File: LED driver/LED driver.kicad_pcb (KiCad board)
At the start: 2 copper layers, 65 x 45 mm, 49 parts, among them J1 Conn_VCC, J2 Conn_LED, J3 Conn_Aux, J4 Conn_UART, J5 PWR_AUX, Q1 ZXMN3A01F, Q2 ZXMN3A01F, Q3 ZXMN3A01F, Q4 ZXMN3A01F, Q5 ZXMN3A01F, SW1 SW_Push, U1 ESP32-C3-MINI-1-N4, U2 MP2359

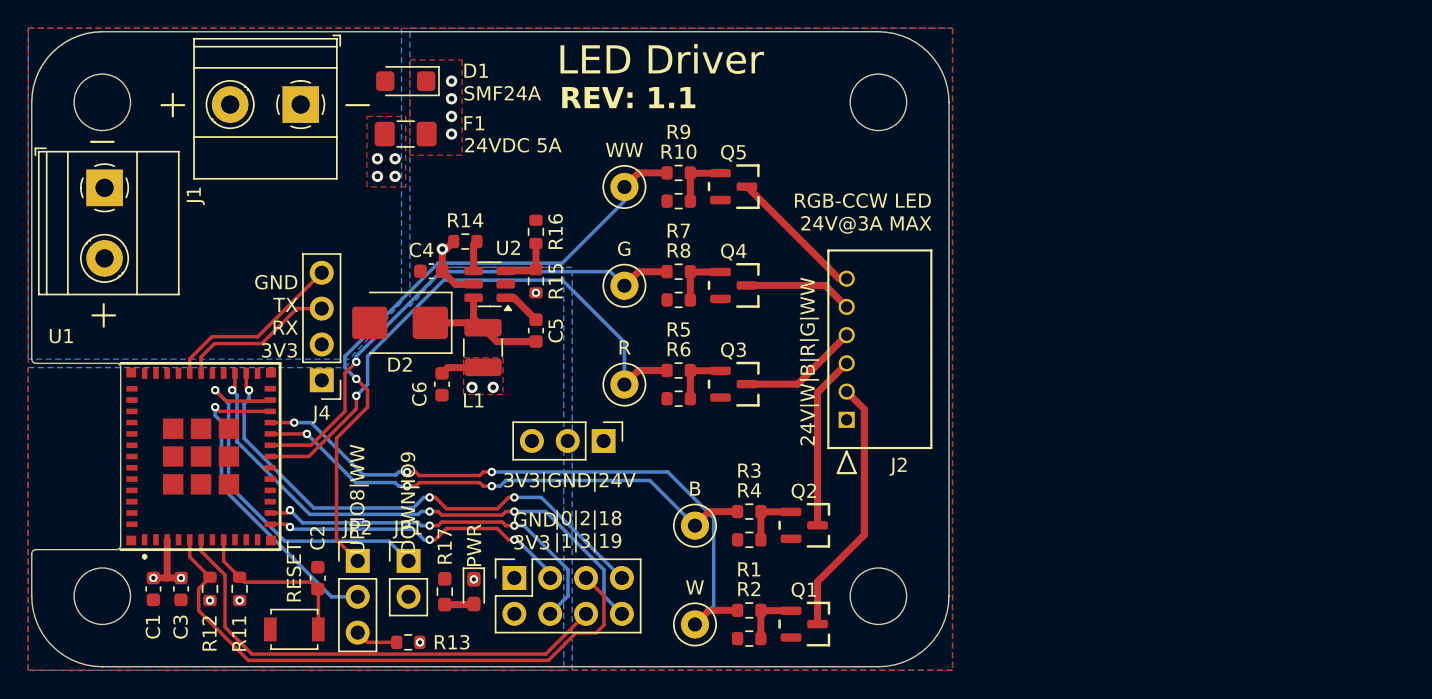
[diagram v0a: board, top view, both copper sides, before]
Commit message: 2024-11-24 (sub-par pcb)
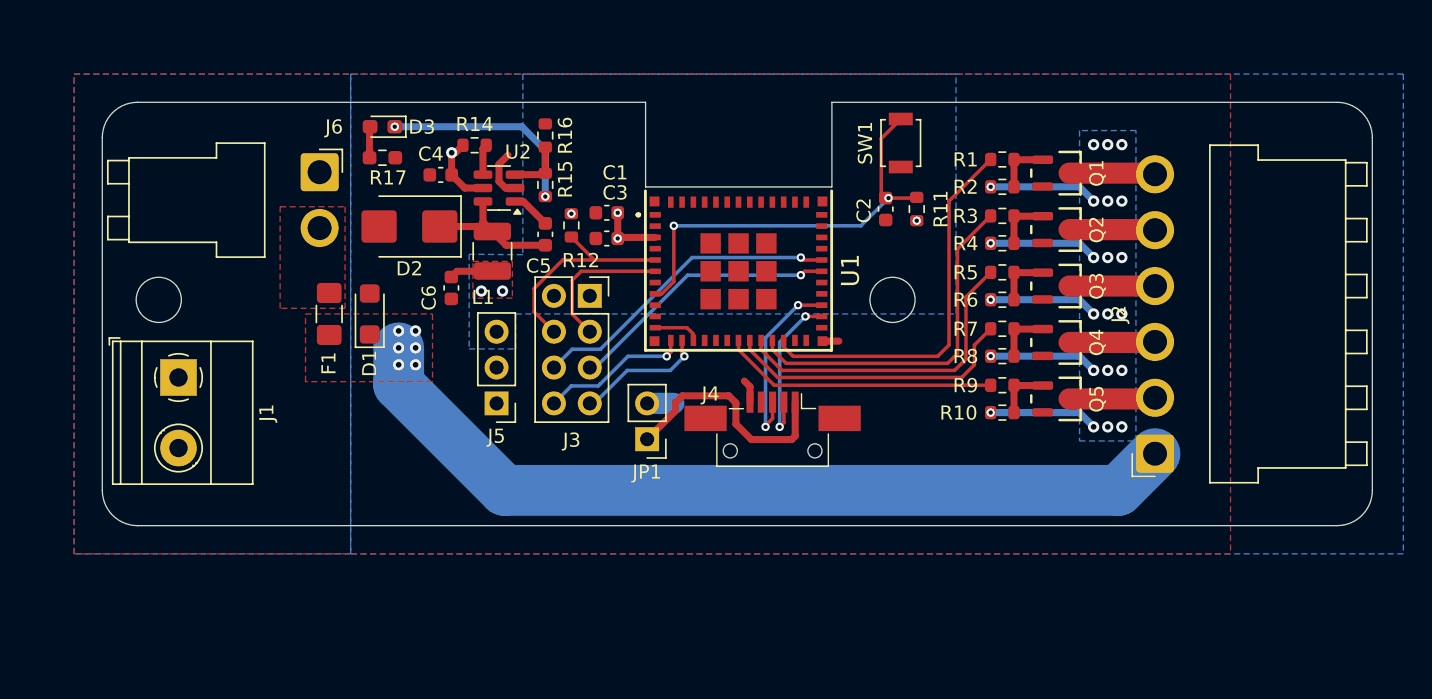
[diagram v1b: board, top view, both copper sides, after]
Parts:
- removed the J1 at (113.9, 57.7)
- removed the J1 at (100.0, 63.6)
- removed JP2: Boot Mode 2, Connector_PinHeader_2.54mm:PinHeader_1x03_P2.54mm_Vertical
- removed R13: 4.7K, Resistor_SMD:R_0603_1608Metric
- removed TP1: PWM_W, TestPoint:TestPoint_Loop_D2.50mm_Drill1.0mm
- removed TP2: PWM_B, TestPoint:TestPoint_Loop_D2.50mm_Drill1.0mm
- removed TP3: PWM_R, TestPoint:TestPoint_Loop_D2.50mm_Drill1.0mm
- removed TP4: PWM_G, TestPoint:TestPoint_Loop_D2.50mm_Drill1.0mm
- removed TP5: PWM_WW, TestPoint:TestPoint_Loop_D2.50mm_Drill1.0mm
- added J1: Conn_VCC_screw, TerminalBlock_Phoenix:TerminalBlock_Phoenix_MKDS-1,5-2_1x02_P5.00mm_Horizontal, F.Cu at (105.2, 77.1)
- added J6: Conn_VCC, Connector_JST:JST_VH_B2PS-VH_1x02_P3.96mm_Horizontal, F.Cu at (115.2, 62.5)
- J2: footprint footprints:CON_532540670_MOL -> Connector_JST:JST_VH_B6PS-VH_1x06_P3.96mm_Horizontal
- J4: value Conn_UART -> USB_B_Mini; footprint Connector_PinHeader_2.54mm:PinHeader_1x04_P2.54mm_Vertical -> Connector_USB:USB_Mini-B_AdamTech_MUSB-B5-S-VT-TSMT-1_SMD_Vertical
- JP1: value Boot Mode 1 -> VBUS_to_VCC
- moved SW1 55.1 mm to (156.4, 60.5), turned to 90 degrees
- moved R11 55.0 mm to (157.5, 65.1)
- moved C2 48.0 mm to (155.3, 65.1), turned to 90 degrees
- moved C1 41.7 mm to (135.6, 65.4), turned to 0 degrees
- moved U1 40.3 mm to (144.9, 69.5), turned to 0 degrees
- moved C3 39.1 mm to (135.6, 67.2), turned to 0 degrees
- moved R2 36.7 mm to (163.6, 63.6)
- moved R1 36.6 mm to (163.6, 61.6)
- moved Q1 36.6 mm to (167.4, 62.6)
- moved R12 36.3 mm to (133.0, 66.3), turned to -90 degrees
- moved D3 33.6 mm to (119.7, 59.3), turned to 180 degrees
- moved J4 32.1 mm to (147.3, 80.4), turned to -90 degrees
- moved R17 31.1 mm to (119.7, 61.5), turned to 180 degrees
- moved R4 27.6 mm to (163.6, 67.6)
- moved R3 27.6 mm to (163.6, 65.6)
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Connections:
- J2 pad 2: /W -> /WW
- J2 pad 3: /B -> /G
- J2 pad 5: /G -> /B
- J2 pad 6: /WW -> /W
- J3 pad 3: /IO0 -> /IO3
- J3 pad 4: /IO1 -> /IO2
- J3 pad 5: /IO2 -> /IO20
- J3 pad 6: /IO3 -> /IO21
- J3 pad 7: /IO18 -> /IO1
- J3 pad 8: /IO19 -> /IO0
- J4 pad 1: +3.3V -> Net-(J4-VBUS)
- J4 pad 2: GND -> /USB_D-
- J4 pad 3: /RX -> /USB_D+
- J4 pad 4: /TX -> unconnected-(J4-ID-Pad4)
- JP1 pad 1: /IO9 -> Net-(J4-VBUS)
- JP1 pad 2: GND -> VCC
- U1 pad 18: /PWM_R -> /PWM_WW
- U1 pad 20: /PWM_B -> /PWM_R
- U1 pad 21: /PWM_W -> /PWM_B
- U1 pad 22: Net-(JP2-C) -> /PWM_W
- U1 pad 23: /IO9 -> unconnected-(U1-IO9-Pad23)
- U1 pad 26: /IO18 -> /USB_D-
- U1 pad 27: /IO19 -> /USB_D+
- U1 pad 30: /RX -> /IO20
- U1 pad 31: /TX -> /IO21
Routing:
- net VCC: track 5.19 -> 67.5 mm, vias 5 -> 7
- net GND: track 0.00 -> 48.2 mm, vias 0 -> 23
- net /IO19: track 38.9 -> 0.00 mm, vias 3 -> 0
- net /IO18: track 37.0 -> 0.00 mm, vias 3 -> 0
- net /IO9: track 26.3 -> 0.00 mm, vias 1 -> 0
- net /PWM_WW: track 45.5 -> 19.6 mm, vias 1 -> 0
- net /IO2: track 41.0 -> 15.4 mm
- net /IO3: track 34.5 -> 10.3 mm
- net Net-(JP2-C): track 22.7 -> 0.00 mm, vias 1 -> 0
- net /IO21: track 0.00 -> 22.3 mm, vias 0 -> 1
- net /IO20: track 0.00 -> 19.3 mm, vias 0 -> 1
- net /PWM_W: track 46.1 -> 27.1 mm, vias 3 -> 0
- net Net-(U1-EN): track 11.9 -> 30.1 mm, vias 0 -> 2
- net /IO1: track 26.8 -> 9.28 mm, vias 3 -> 1
- net /PWM_R: track 40.3 -> 23.0 mm, vias 1 -> 0
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- added copper zone on B.Cu, net GND
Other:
- board size 65 x 45 mm -> 90 x 30 mm
- board text removed: "+24V"
- board text removed: "+24V (fused)"
- board text removed: "+24V (no fuse)"
- board text removed: "+3V3"
- board text removed: "2024-09-01"
- board text removed: "24V|W|B|R|G|WW"
- board text removed: "3V3|GND|24V"
- board text removed: "<CodedSakura/>"
- board text removed: "=4mm =65mm =55mm =45mm =35mm"
- board text removed: "B"
- board text removed: "DOWN|IO9"
- board text removed: "G"
- board text removed: "GND"
- board text removed: "GND 3V3"
- board text removed: "GND TX RX 3V3"
- board text removed: "JLCJLCJLCJLC"
- board text removed: "LED Driver"
- board text removed: "PWR"
- board text removed: "R"
- board text removed: "RESET"
- board text removed: "REV: 1.1"
- board text removed: "RGB-CCW LED 24V@3A MAX"
- board text removed: "UP|IO8|WW"
- board text removed: "W"
- board text removed: "WW"
- board text removed: "h"
- board text removed: "w"
- board text removed: "w x h y"
- board text removed: "x"
- board text removed: "y"
- board text removed: "|0|2|18 |1|3|19"
